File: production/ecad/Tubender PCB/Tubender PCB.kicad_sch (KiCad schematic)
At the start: 0 parts

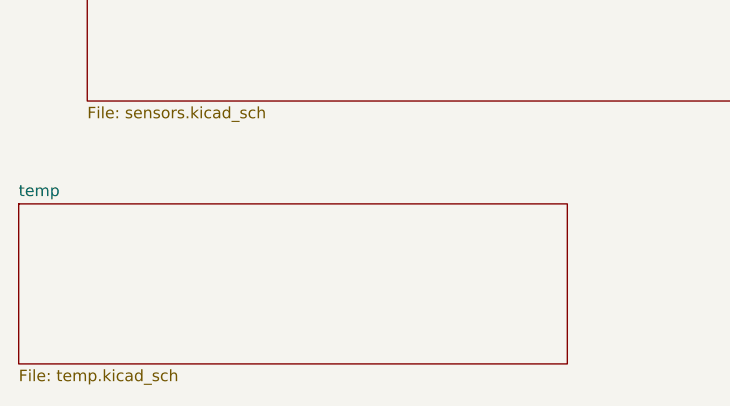
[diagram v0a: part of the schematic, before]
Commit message: final for rev 1
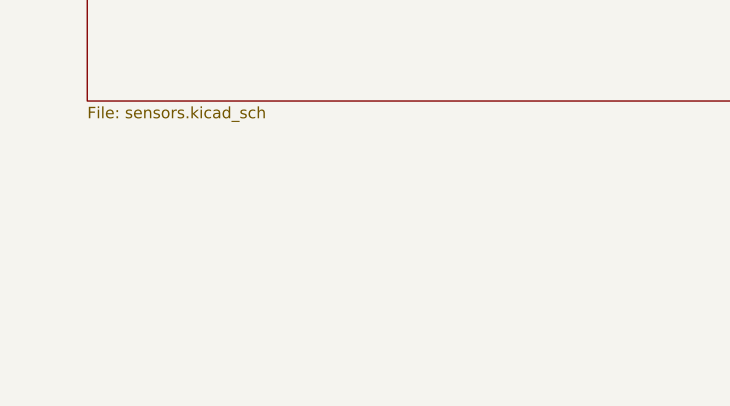
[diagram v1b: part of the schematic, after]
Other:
- removed sheet temp
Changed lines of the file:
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@@
-	)
-	(sheet
-		(at 43.18 173.99)
-		(size 60.96 17.78)
-		(fields_autoplaced yes)
-		(stroke
-			(width 0.1524)
-			(type solid)
-		)
-		(fill
-			(color 0 0 0 0.0000)
-		)
-		(property "Sheetname" "temp"
-			(at 43.18 173.2784 0)
-			(effects
-				(font
-					(size 1.27 1.27)
-				)
-				(justify left bottom)
-			)
-		)
-		(property "Sheetfile" "temp.kicad_sch"
-			(at 43.18 192.3546 0)
-			(effects
-				(font
-					(size 1.27 1.27)
-				)
-				(justify left top)
-			)
-		)
-		(instances
-			(project "Tubender PCB"
-				(path "/3e1aedd0-6089-4edb-92c7-0c31da2e7927"
-					(page "7")
-				)
-			)
-		)
 	)
 	(sheet
